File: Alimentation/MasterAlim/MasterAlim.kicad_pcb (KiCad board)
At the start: 4 copper layers, 85 x 42.8 mm, 53 parts, among them J1 Ext-Con, J10 Reg Log, J11 AU Logic, J12 INHIBIT, J13 ToRegul, J2 Alim logique, J3 Batt IN, J4 INHIBIT, J5 ToRegul, J6 INHIBIT, J7 ToRegul, J8 INHIBIT, J9 ToRegul, U1 74LVC1G02, U2 74LVC1G02, U3 74LVC1G02, U4 74LVC1G02, U8 PCF8574A

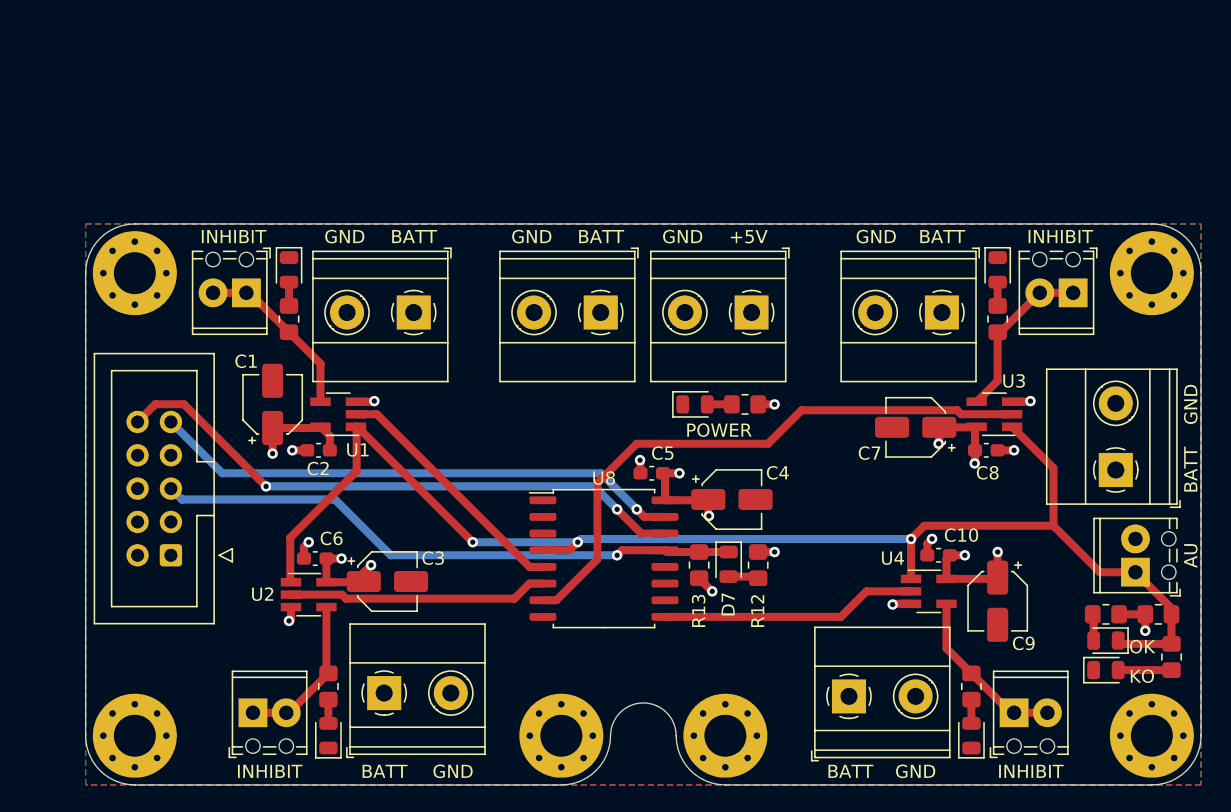
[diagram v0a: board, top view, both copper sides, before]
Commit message: Rework suite point robot
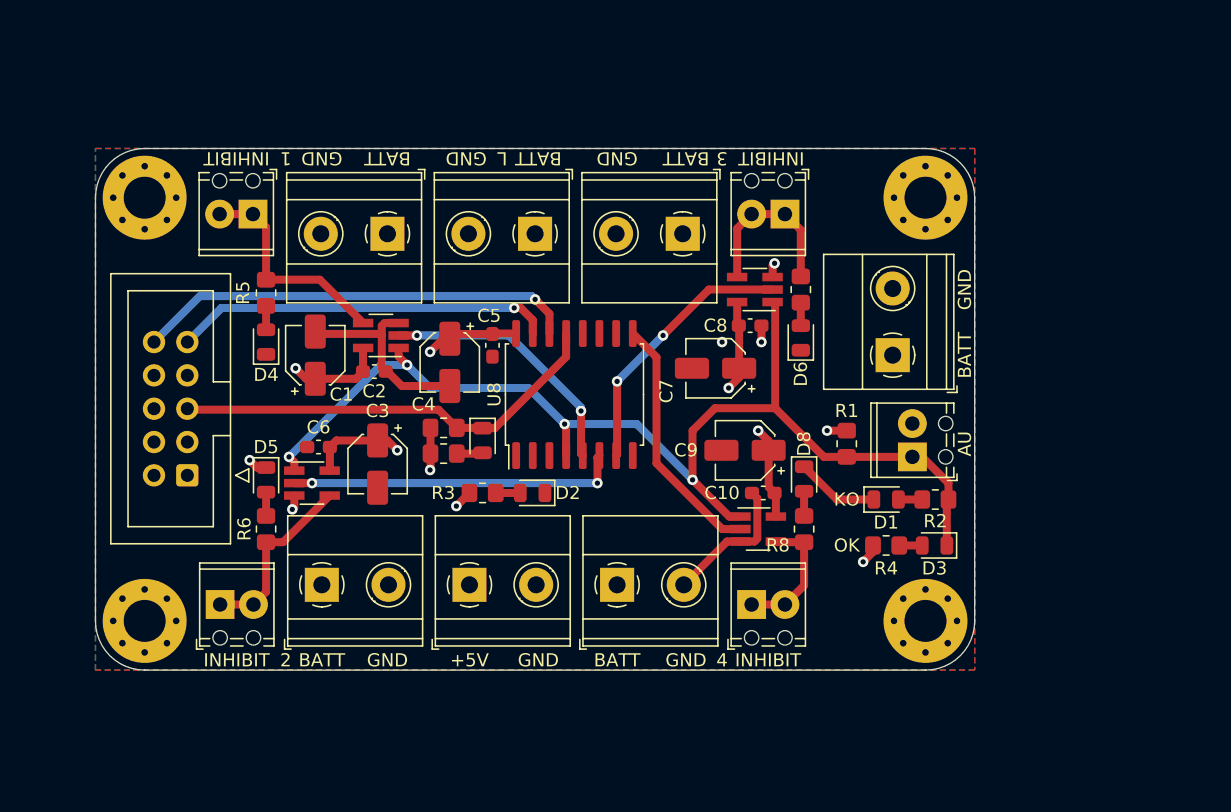
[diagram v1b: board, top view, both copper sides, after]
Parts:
- removed H6, H7, H8: MountingHole_Pad, MountingHole:MountingHole_3.2mm_M3_Pad_Via
- added H3: MountingHole_Pad, MountingHole:MountingHole_3.2mm_M3_Pad_Via, F.Cu at (164.0, 48.0)
- moved J2 29.9 mm to (129.2, 77.5), turned to 0 degrees
- moved H4 29.1 mm to (164.0, 80.2)
- moved R1 27.1 mm to (158.0, 66.8), turned to 270 degrees
- moved R12 25.4 mm to (127.3, 67.5), turned to 0 degrees
- moved C4 23.9 mm to (127.8, 60.5), turned to 270 degrees
- moved D8 23.4 mm to (154.8, 69.4), turned to 270 degrees
- moved J8 22.8 mm to (153.3, 49.2)
- moved C9 22.4 mm to (150.2, 67.2), turned to 180 degrees
- moved R13 22.1 mm to (127.3, 65.5), turned to 0 degrees
- moved J12 21.6 mm to (150.8, 79.0)
- moved R2 21.6 mm to (164.8, 71.0), turned to 180 degrees
- moved D1 21.2 mm to (161.0, 71.0)
- moved R3 21.1 mm to (130.2, 70.5), turned to 0 degrees
- moved D7 21.0 mm to (130.2, 66.5)
- moved J9 20.6 mm to (145.5, 50.8)
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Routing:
- net GND: track 11.6 -> 37.5 mm, vias 9 -> 5
- net /PIL_T3: track 45.3 -> 20.4 mm, vias 0 -> 2
- net /AU: track 104.6 -> 86.6 mm, vias 3 -> 4
- net SDA: track 40.6 -> 28.8 mm
- net /IRQ: track 44.8 -> 33.5 mm, vias 1 -> 0
- net SCL: track 44.8 -> 33.6 mm, vias 2 -> 1
- net /PIL_T2: track 19.8 -> 25.3 mm, vias 0 -> 2
- net /PilAlim1/Y: track 13.3 -> 16.7 mm
- net /sheet602E5F6A/Y: track 13.1 -> 10.1 mm
- net Net-(D1-Pad2): track 4.06 -> 1.81 mm
- net +5V: track 46.1 -> 43.8 mm, vias 13 -> 9
- net /sheet602E5506/Y: track 12.1 -> 14.0 mm
- net /PIL_T1: track 19.1 -> 19.9 mm, vias 0 -> 2
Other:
- board size 85 x 42.8 mm -> 67 x 39.8 mm
- board text added: "1"
- board text added: "2"
- board text added: "3"
- board text added: "4"
- board text added: "L"
- board text removed: "POWER"

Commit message: Finalisation alimentations
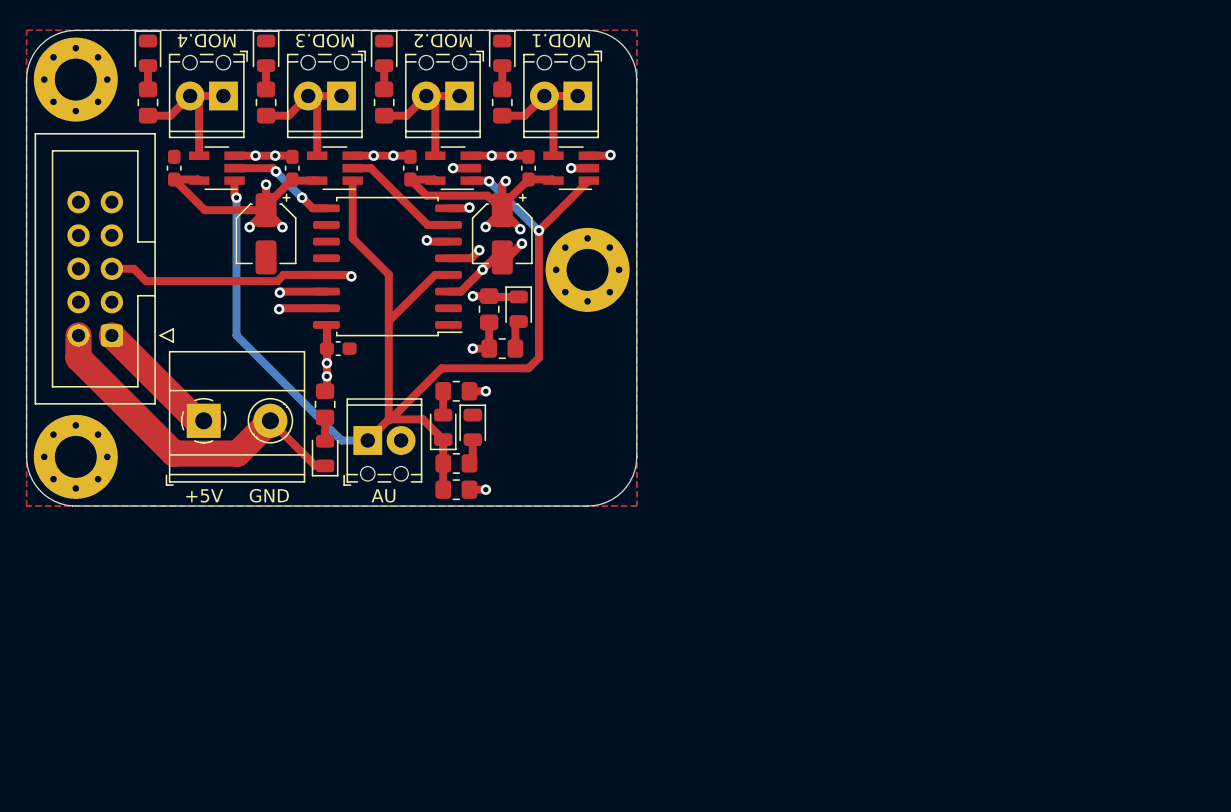
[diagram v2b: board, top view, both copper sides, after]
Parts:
- removed C4, C7, C9: 1u, Capacitor_SMD:CP_Elec_4x5.3
- removed H4: MountingHole_Pad, MountingHole:MountingHole_3.2mm_M3_Pad_Via
- removed J10: Reg Log, TerminalBlock_Phoenix:TerminalBlock_Phoenix_MKDS-1,5-2-5.08_1x02_P5.08mm_Horizontal
- removed J13, J5, J7, J9: ToRegul, TerminalBlock_Phoenix:TerminalBlock_Phoenix_MKDS-1,5-2-5.08_1x02_P5.08mm_Horizontal
- removed J3: Batt IN, TerminalBlock_Phoenix:TerminalBlock_Phoenix_MKDS-1,5-2-5.08_1x02_P5.08mm_Horizontal
- moved R8 59.6 mm to (104.8, 40.8)
- moved D8 59.6 mm to (104.8, 37.0)
- moved J12 55.9 mm to (110.5, 40.2), turned to 180 degrees
- moved C10 51.3 mm to (106.8, 45.8), turned to 90 degrees
- moved U4 49.6 mm to (110.0, 45.8), turned to 180 degrees
- moved D6 46.2 mm to (113.8, 37.0), turned to 270 degrees
- moved R7 43.2 mm to (113.8, 40.8), turned to 90 degrees
- moved J6 42.8 mm to (128.5, 40.2), turned to 180 degrees
- moved J11 41.5 mm to (121.5, 66.5), turned to 0 degrees
- moved D3 38.5 mm to (127.2, 65.5), turned to 90 degrees
- moved C8 36.9 mm to (115.8, 45.8), turned to 90 degrees
- moved R2 36.6 mm to (128.2, 68.2), turned to 0 degrees
- moved J8 35.0 mm to (119.5, 40.2)
- moved R4 34.8 mm to (128.2, 62.8), turned to 180 degrees
- moved D5 33.7 mm to (122.8, 37.0)
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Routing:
- net +5V: track 43.8 -> 62.2 mm, vias 9 -> 11
- net /PIL_T2: track 25.3 -> 9.37 mm
- net GND: track 37.5 -> 49.7 mm, vias 5 -> 10
- net /PIL_T3: track 20.4 -> 9.09 mm, vias 2 -> 0
- net /PIL_T4: track 19.1 -> 8.27 mm, vias 0 -> 2
- net SCL: track 33.6 -> 22.9 mm
- net /AU: track 86.6 -> 96.6 mm, vias 4 -> 3
- net SDA: track 28.8 -> 19.8 mm
- net /PIL_T1: track 19.9 -> 13.5 mm
- net /PilAlim1/Y: track 16.7 -> 11.2 mm
- net /sheet602E5506/Y: track 14.0 -> 11.2 mm
- net /sheet602E5F64/Y: track 13.0 -> 11.2 mm
- net /IRQ: track 33.5 -> 32.3 mm, vias 0 -> 2
- net /sheet602E5F6A/Y: track 10.1 -> 11.2 mm
- added copper zone on In2.Cu, net +5V
- removed copper zone on In1.Cu, net +5V
- removed copper zone on In2.Cu, net +BATT
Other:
- board size 67 x 39.8 mm -> 46.5 x 36.2 mm
- board text added: "MOD.1"
- board text added: "MOD.2"
- board text added: "MOD.3"
- board text added: "MOD.4"
- board text removed: "1"
- board text removed: "2"
- board text removed: "3"
- board text removed: "4"
- board text removed: "BATT"
- board text removed: "INHIBIT"
- board text removed: "KO"
- board text removed: "L"
- board text removed: "OK"
